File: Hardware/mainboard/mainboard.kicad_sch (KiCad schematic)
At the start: 25 parts, among them J1 Conn_01x18_Pin, J2 Conn_01x11_Pin, J3 Conn_01x04_Pin, J4 USB_B_Micro, SW1 SW_SPDT, U1 STM32L151CBTxA, U2 AMS1117-3.3, Y1 16MHz

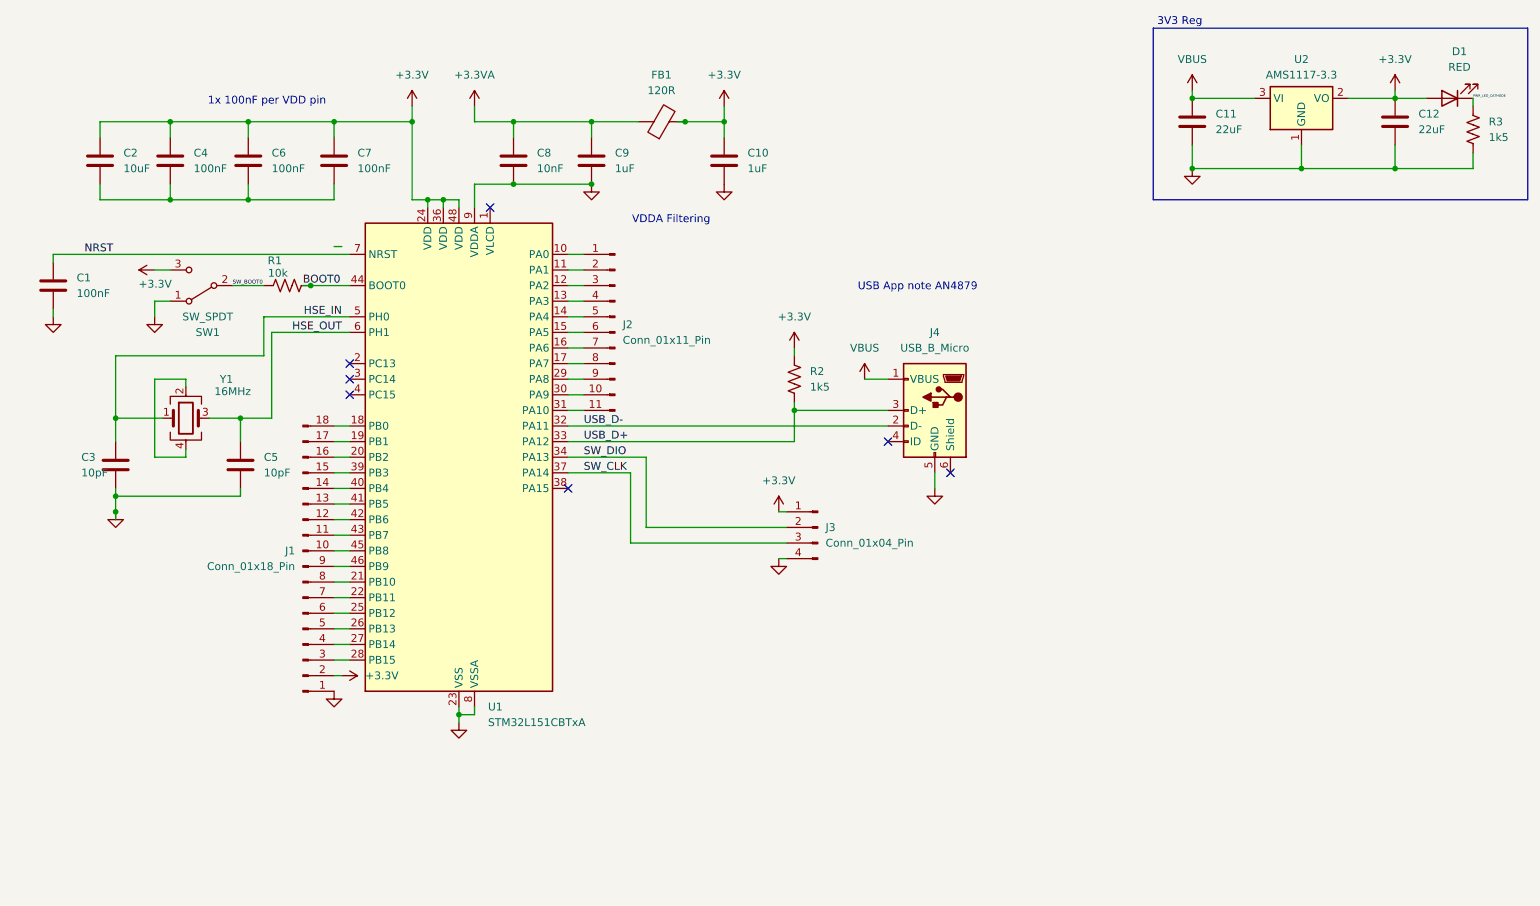
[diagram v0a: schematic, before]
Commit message: more work on pcb
finished house season 2 and made decent progress (i think) on the pcb. if it is bad ill see tomorrow lol
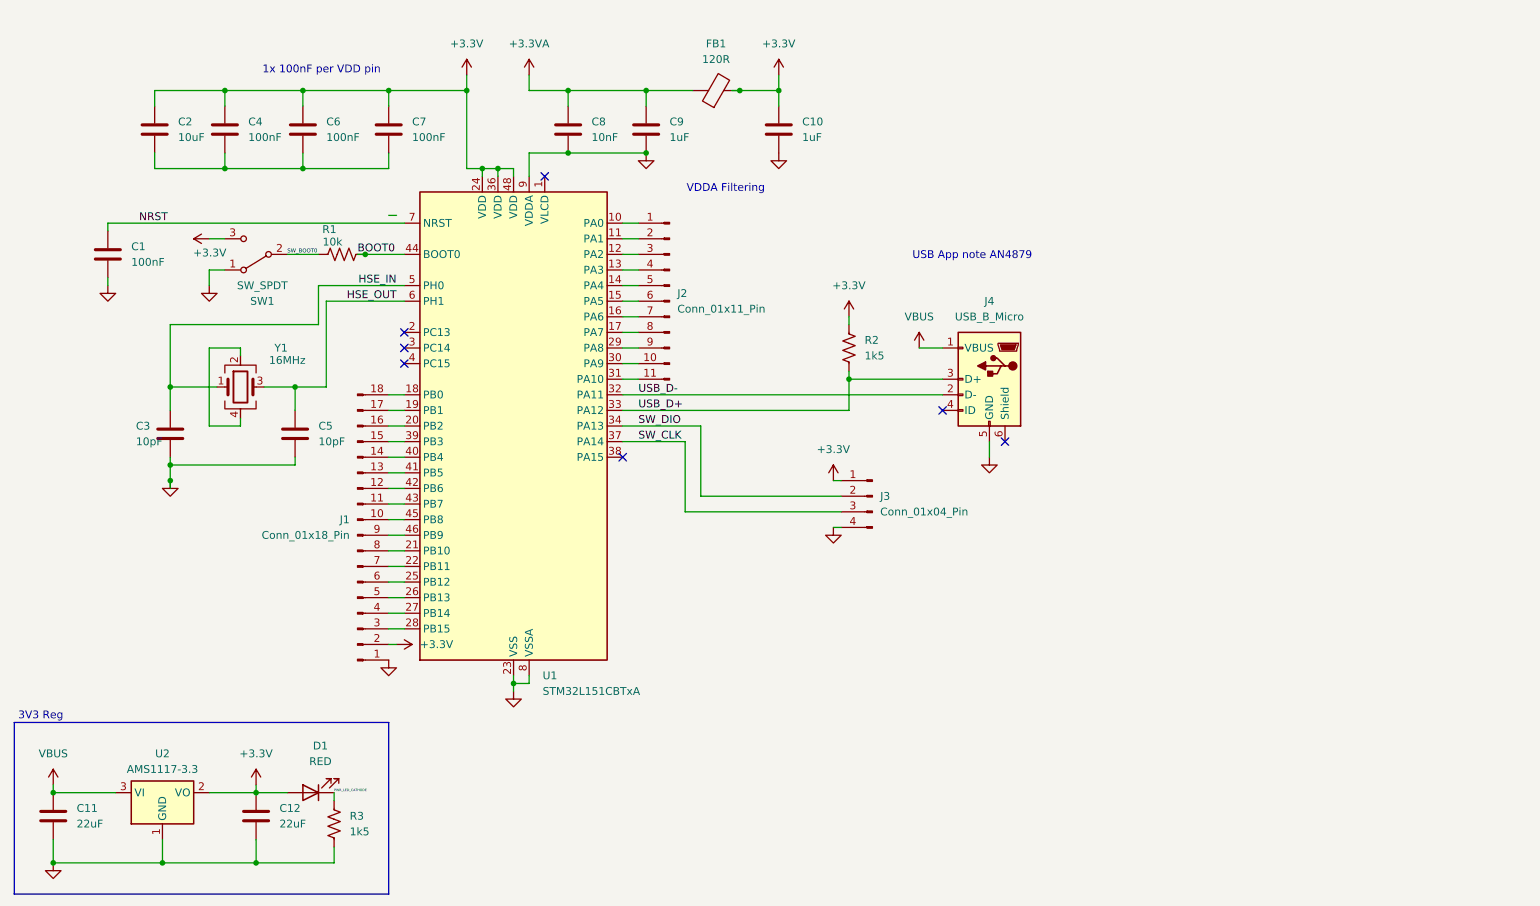
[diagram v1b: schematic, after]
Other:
- title: (none) -> L151 breakout board
- moved on the sheet: C1, C10, C11, C12, C2, C3, C4, C5, C6, C7, C8, C9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
